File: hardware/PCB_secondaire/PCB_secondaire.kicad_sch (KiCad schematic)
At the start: 13 parts, among them J1 Conn_01x07, J2 Conn_01x06, J3 Conn_01x07, J4 Conn_01x07, J5 Conn_01x07, J6 Conn_01x07, J7 Conn_01x06, J8 Conn_01x06, J9 Conn_01x07

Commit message: PCBs v2
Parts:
- J3, J4, J5: footprint Connector_PinHeader_2.54mm:PinHeader_1x07_P2.54mm_Vertical -> Connector_PinHeader_2.54mm:PinHeader_1x07_P2.54mm_Horizontal
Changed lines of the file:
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@@
 			)
 		)
-		(property "Footprint" "Connector_PinHeader_2.54mm:PinHeader_1x07_P2.54mm_Vertical"
+		(property "Footprint" "Connector_PinHeader_2.54mm:PinHeader_1x07_P2.54mm_Horizontal"
 			(at 158.75 115.57 0)
 			(effects
@@
 			)
 		)
-		(property "Footprint" "Connector_PinHeader_2.54mm:PinHeader_1x07_P2.54mm_Vertical"
+		(property "Footprint" "Connector_PinHeader_2.54mm:PinHeader_1x07_P2.54mm_Horizontal"
 			(at 120.65 115.57 0)
 			(effects
@@
 			)
 		)
-		(property "Footprint" "Connector_PinHeader_2.54mm:PinHeader_1x07_P2.54mm_Vertical"
+		(property "Footprint" "Connector_PinHeader_2.54mm:PinHeader_1x07_P2.54mm_Horizontal"
 			(at 158.75 92.71 0)
 			(effects

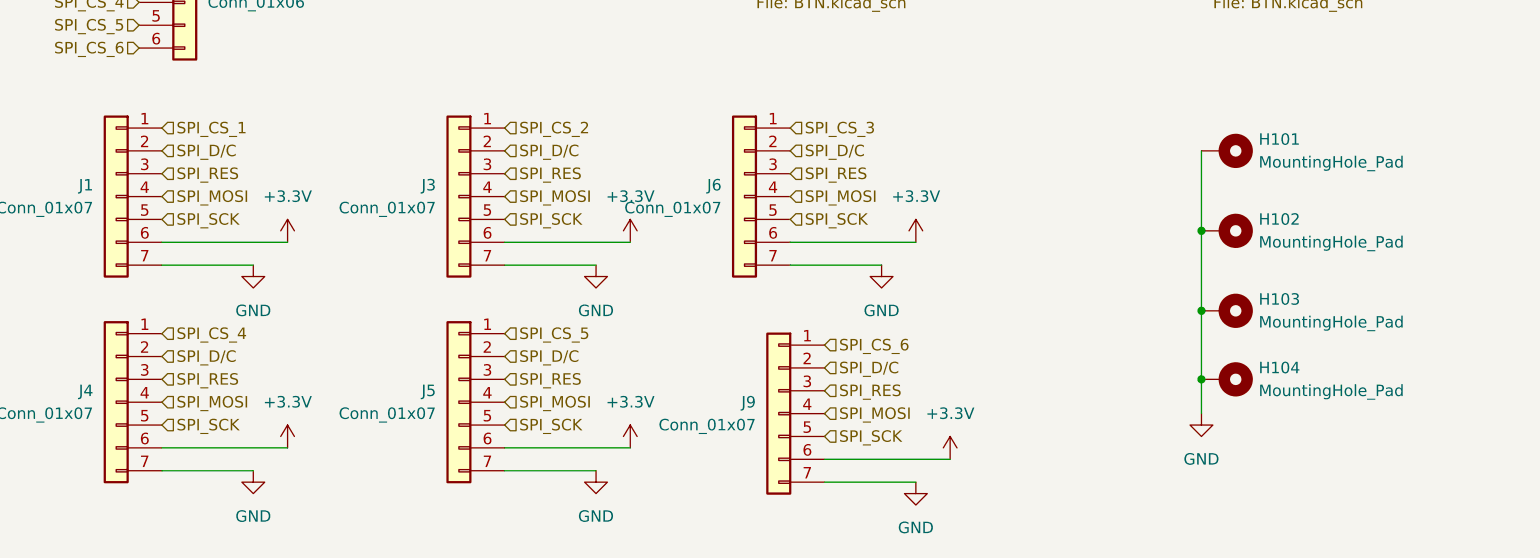
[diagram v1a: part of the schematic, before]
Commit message: PCBs v3
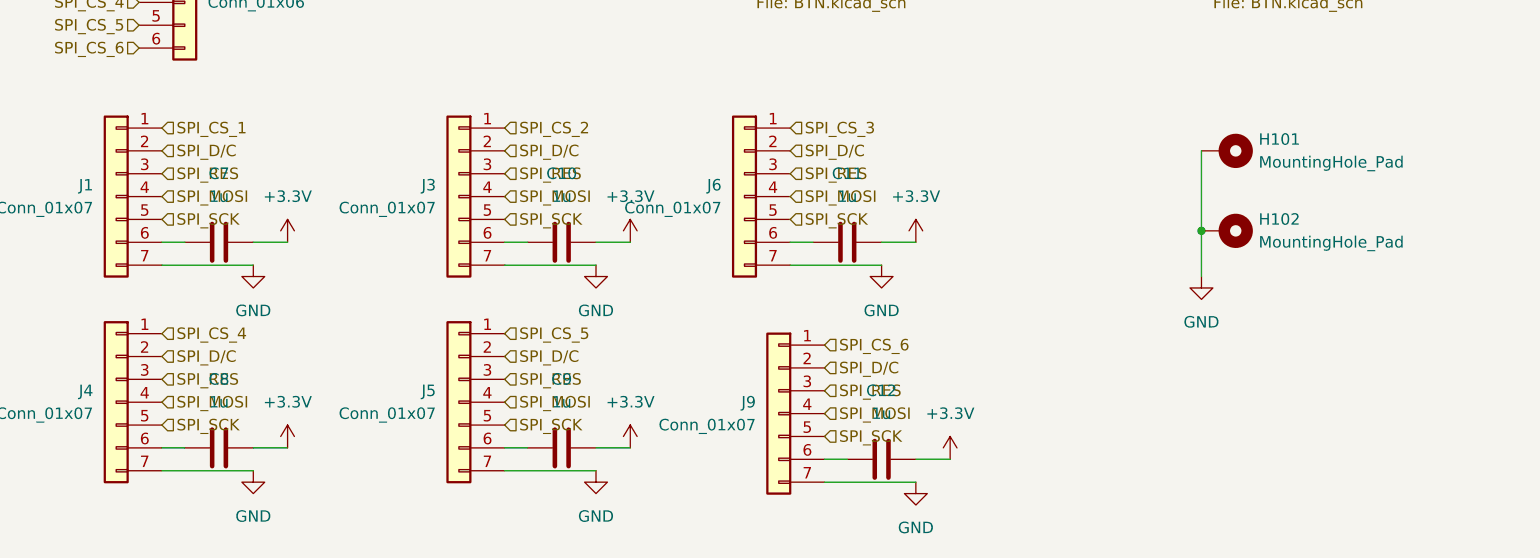
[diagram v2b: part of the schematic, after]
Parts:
- removed H103, H104: MountingHole_Pad, MountingHole:MountingHole_3.2mm_M3_Pad_Via, symbol Mechanical:MountingHole_Pad
- added C10, C11, C12, C7, C8, C9: 1u, Capacitor_SMD:C_0603_1608Metric, symbol Device:C
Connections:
- net +3.3V: now also C10.2, C11.2, C12.2, C7.2, C8.2, C9.2; no longer J1.6 (Pin_6), J3.6 (Pin_6), J4.6 (Pin_6), J5.6 (Pin_6), J6.6 (Pin_6), J9.6 (Pin_6)
- new net: C11.1, J6.6 (Pin_6)
- new net: C9.1, J5.6 (Pin_6)
- new net: C12.1, J9.6 (Pin_6)
- new net: C8.1, J4.6 (Pin_6)
- new net: C7.1, J1.6 (Pin_6)
- new net: C10.1, J3.6 (Pin_6)

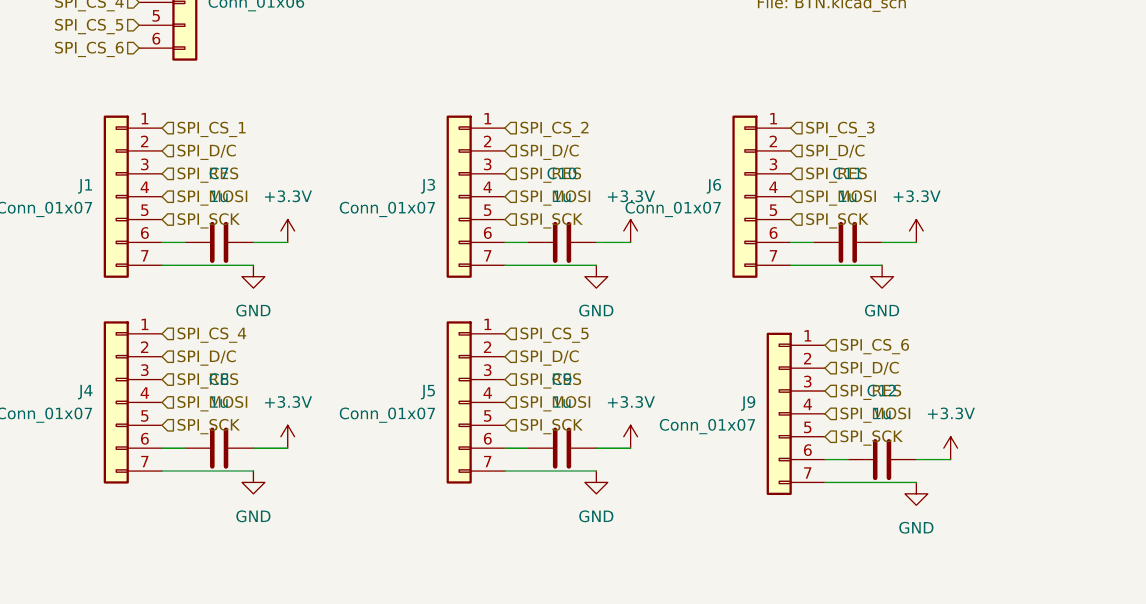
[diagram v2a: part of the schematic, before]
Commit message: PCBs v4
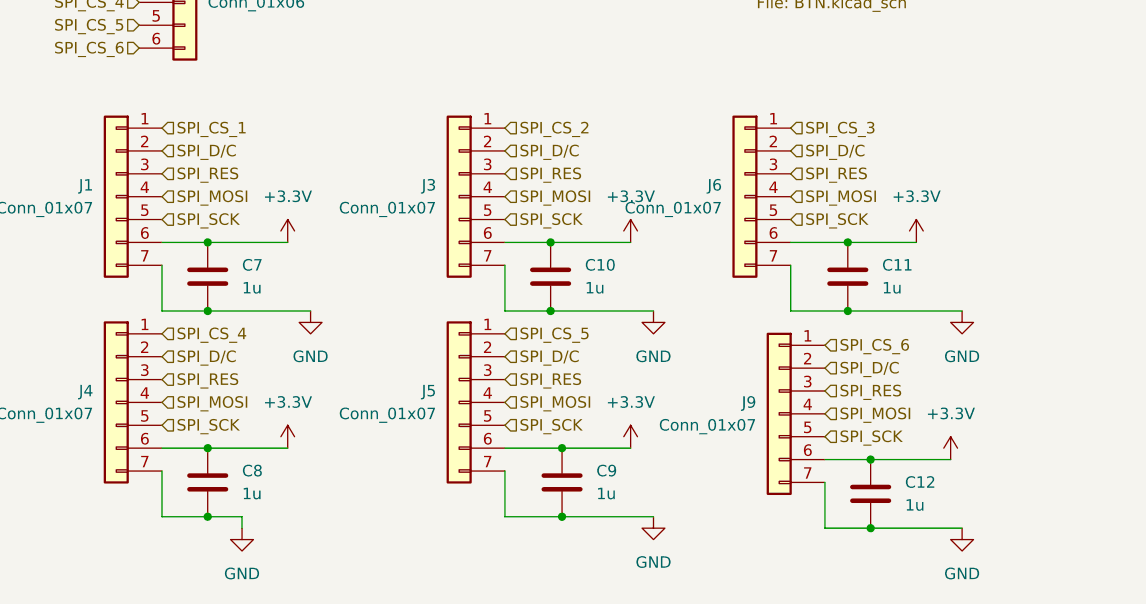
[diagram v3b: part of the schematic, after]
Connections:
- net +3.3V: now also J1.6 (Pin_6), J3.6 (Pin_6), J4.6 (Pin_6), J5.6 (Pin_6), J6.6 (Pin_6), J9.6 (Pin_6)
- net GND: now also C10.1, C11.1, C12.1, C7.1, C8.1, C9.1
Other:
- moved on the sheet: C10, C11, C12, C7, C8, C9
